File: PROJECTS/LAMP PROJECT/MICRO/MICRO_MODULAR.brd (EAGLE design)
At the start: 142.2 x 123.2 mm, 36 parts, among them J1 1X8, J2 1X8

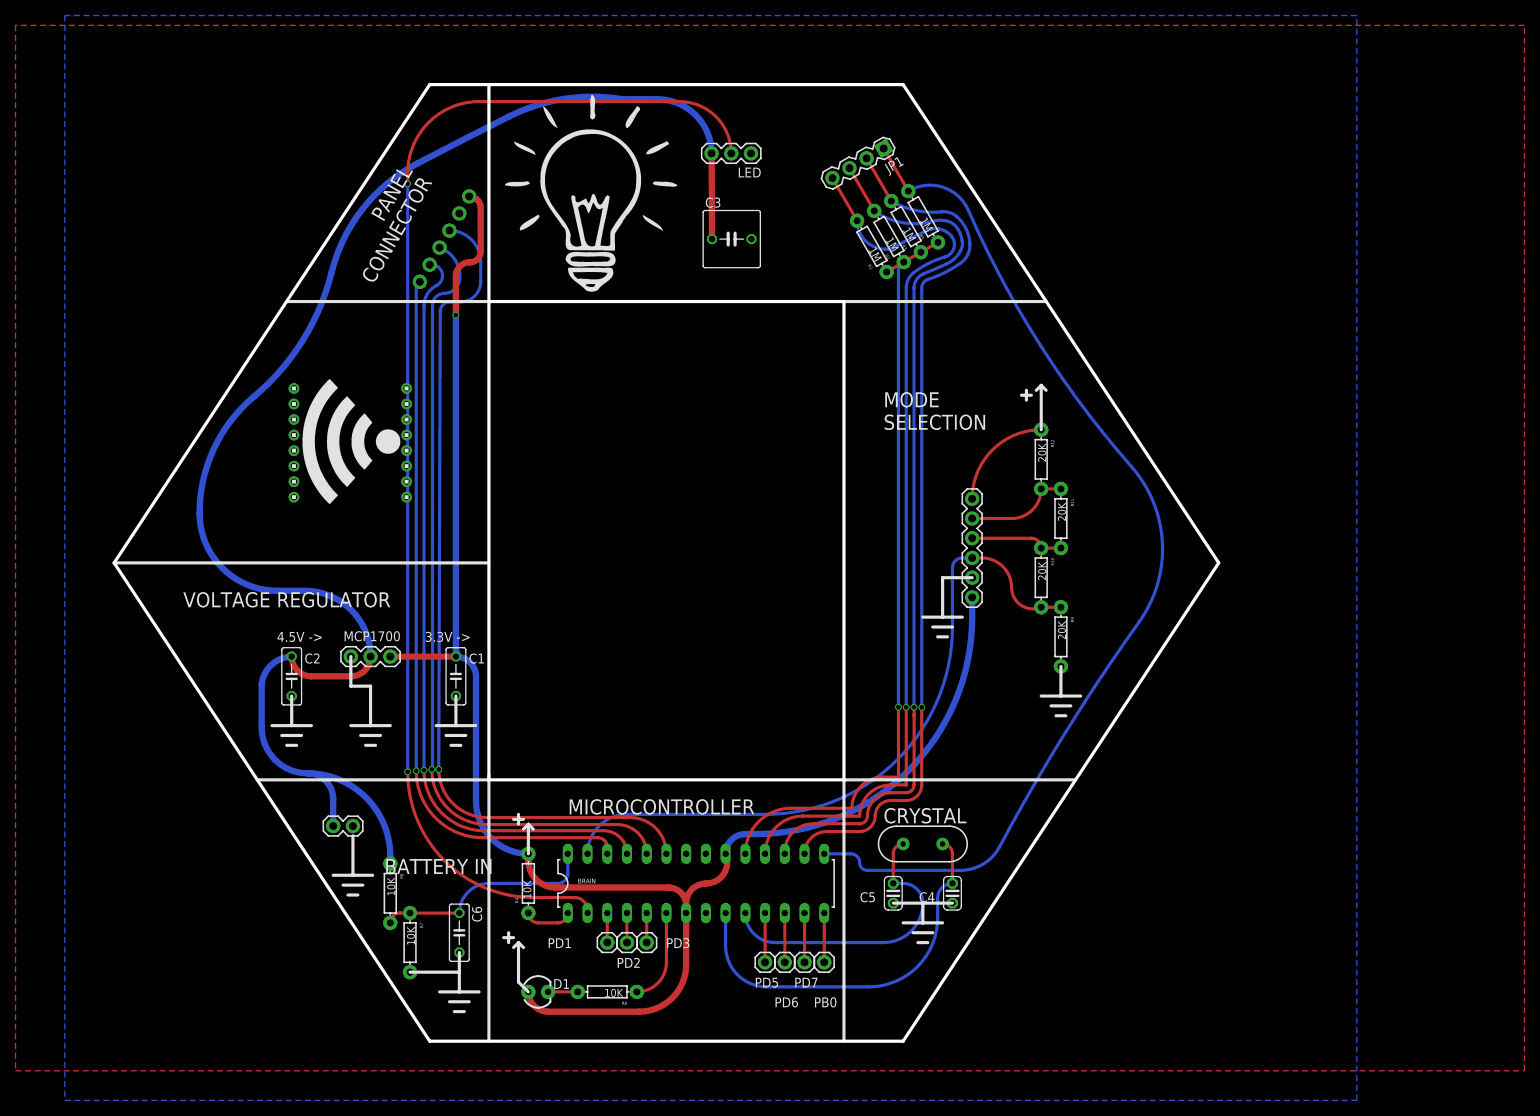
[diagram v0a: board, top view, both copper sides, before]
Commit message: updates to lamp project
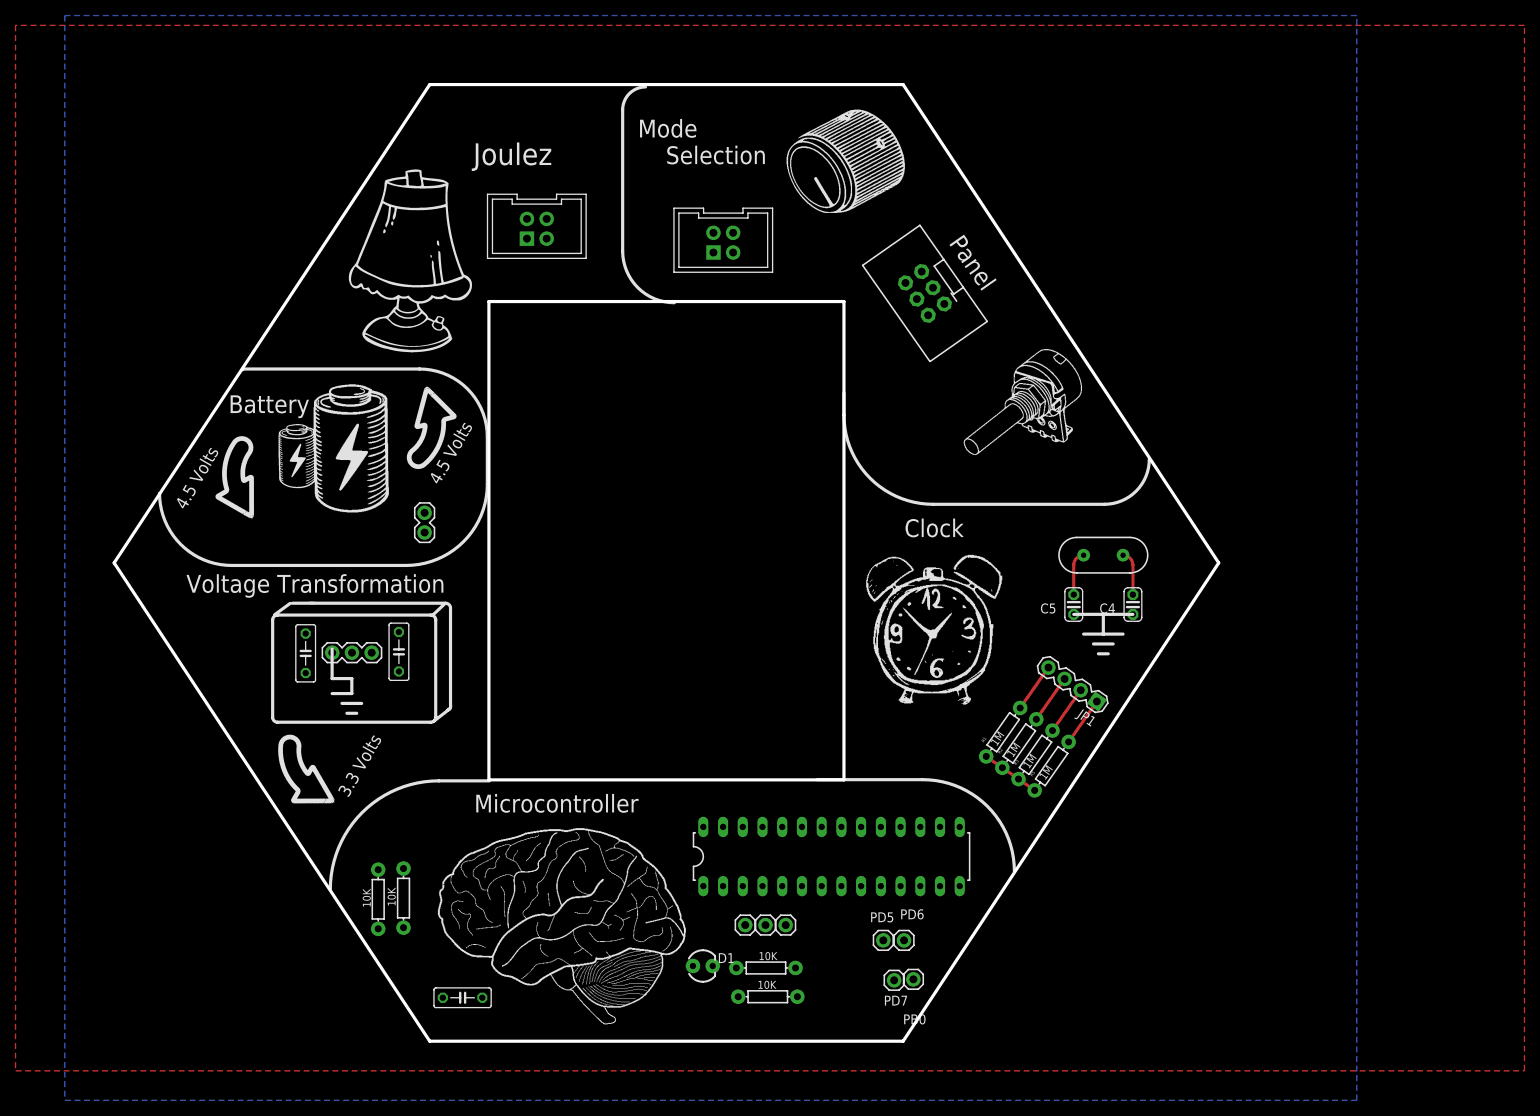
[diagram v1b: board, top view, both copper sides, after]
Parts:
- removed C3: 1000uF, adafruit:C050-075X075
- removed J1, J2: 1X8, RodrigoMarques_Parts:1X8
- removed MODE: (no value), SparkFun-Connectors:1X06
- removed R10, R11, R12, R9: 20K, SparkFun-Passives:AXIAL-0.3
- added LED1: M2X2, RodrigoMarques_Parts:2X2
- LED: value (none) -> M2X2; device SparkFun-Connectors:1X03 -> RodrigoMarques_Parts:2X2
- PANEL: device SparkFun-Connectors:1X06_NO_SILK -> SparkFun-Connectors:2X3-SHROUDED
- moved JP1 76.3 mm to (126.6, 43.7), turned to 145 degrees
- moved R5 72.7 mm to (120.7, 35.4), turned to 55 degrees
- moved R3 70.0 mm to (118.6, 36.9), turned to 55 degrees
- moved R2 67.4 mm to (116.6, 38.3), turned to 55 degrees
- moved PANEL 65.1 mm to (104.4, 96.3), turned to 215 degrees
- moved R1 64.8 mm to (114.5, 39.8), turned to 55 degrees
- moved C4 43.9 mm to (131.2, 56.2)
- moved C5 43.9 mm to (123.6, 56.2)
- moved CRYSTAL 43.9 mm to (127.4, 62.6)
- moved ON_OFF 38.9 mm to (40.0, 65.5), turned to 90 degrees
- moved R4 34.1 mm to (84.2, 5.73), turned to 0 degrees
- moved LED 30.1 mm to (53.2, 105.9), turned to 0 degrees
- moved D1 21.5 mm to (75.8, 9.69)
- moved R8 20.7 mm to (83.9, 9.43)
- moved PD3 18.0 mm to (86.5, 15.0)
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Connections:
- removed net N$19: MODE.6, R12.P$1
- removed net N$20: MODE.5, R11.P$1, R12.P$2
- removed net N$21: MODE.4, R10.P$1, R11.P$2
- net GND: now also LED.PIN1, LED.PIN4, LED1.PIN1, LED1.PIN4; no longer C3.2, LED.1, MODE.2, R9.P$2
- net LEDS_BRAIN: now also LED.PIN2; no longer LED.2
- net N$13: now also LED1.PIN2; no longer MODE.3, R10.P$2, R9.P$1
- net SWITCH_BRAIN: now also LED.PIN3; no longer C3.1, LED.3
- net V_5V: now also LED1.PIN3; no longer MODE.1
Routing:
- net V_5V: track 209.4 -> 0.00 mm, vias 1 -> 0
- net SWITCH_BRAIN: track 192.0 -> 0.00 mm
- net LEDS_BRAIN: track 156.2 -> 0.00 mm, vias 2 -> 0
- net N$2: track 132.0 -> 6.35 mm
- net N$5: track 116.2 -> 6.35 mm, vias 1 -> 0
- net SPEED_BRAIN: track 107.9 -> 0.00 mm, vias 1 -> 0
- net N$4: track 112.8 -> 6.35 mm, vias 1 -> 0
- net N$3: track 110.5 -> 6.35 mm, vias 1 -> 0
- net GREEN_BRAIN: track 101.7 -> 0.00 mm, vias 1 -> 0
- net BLUE_BRAIN: track 96.3 -> 0.00 mm, vias 1 -> 0
- net RED_BRAIN: track 92.7 -> 0.00 mm, vias 1 -> 0
- net N$6: track 98.0 -> 7.62 mm, vias 1 -> 0
- net N$13: track 83.6 -> 0.00 mm
- net N$7: track 48.3 -> 5.61 mm
- net N$8: track 37.0 -> 5.61 mm
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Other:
- outline, holes or cut-outs redrawn
- board text added: "3.3 Volts"
- board text added: "4.5 Volts"
- board text added: "Battery"
- board text added: "Clock"
- board text added: "Joulez"
- board text added: "Microcontroller"
- board text added: "Mode Selection"
- board text added: "Panel"
- board text added: "Voltage Transformation"
- board text removed: "3.3V ->"
- board text removed: "4.5V ->"
- board text removed: "BATTERY IN"
- board text removed: "MICROCONTROLLER"
- board text removed: "MODE SELECTION"
- board text removed: "PANEL CONNECTOR"
- board text removed: "VOLTAGE REGULATOR"
